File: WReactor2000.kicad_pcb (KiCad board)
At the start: 4 copper layers, 63 x 62.2 mm, 32 parts, among them Q1 BSC026N08NS, U1 LTC4359-MS8, U2 ET60T-02-24-02-X-RTX-GP, U4 TM4C1230H6PM, U6 LTC3604_UD, U7 LTC3604_UD

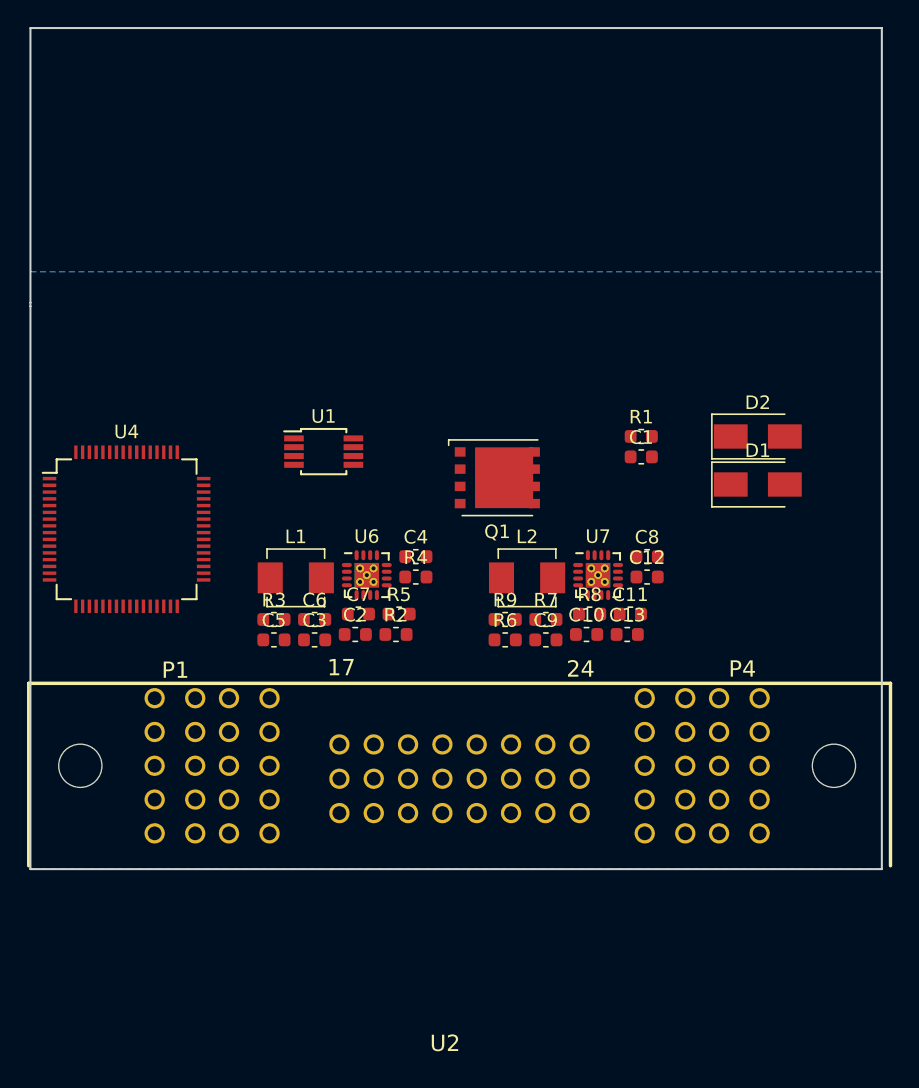
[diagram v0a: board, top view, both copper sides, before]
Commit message: dumb-updates
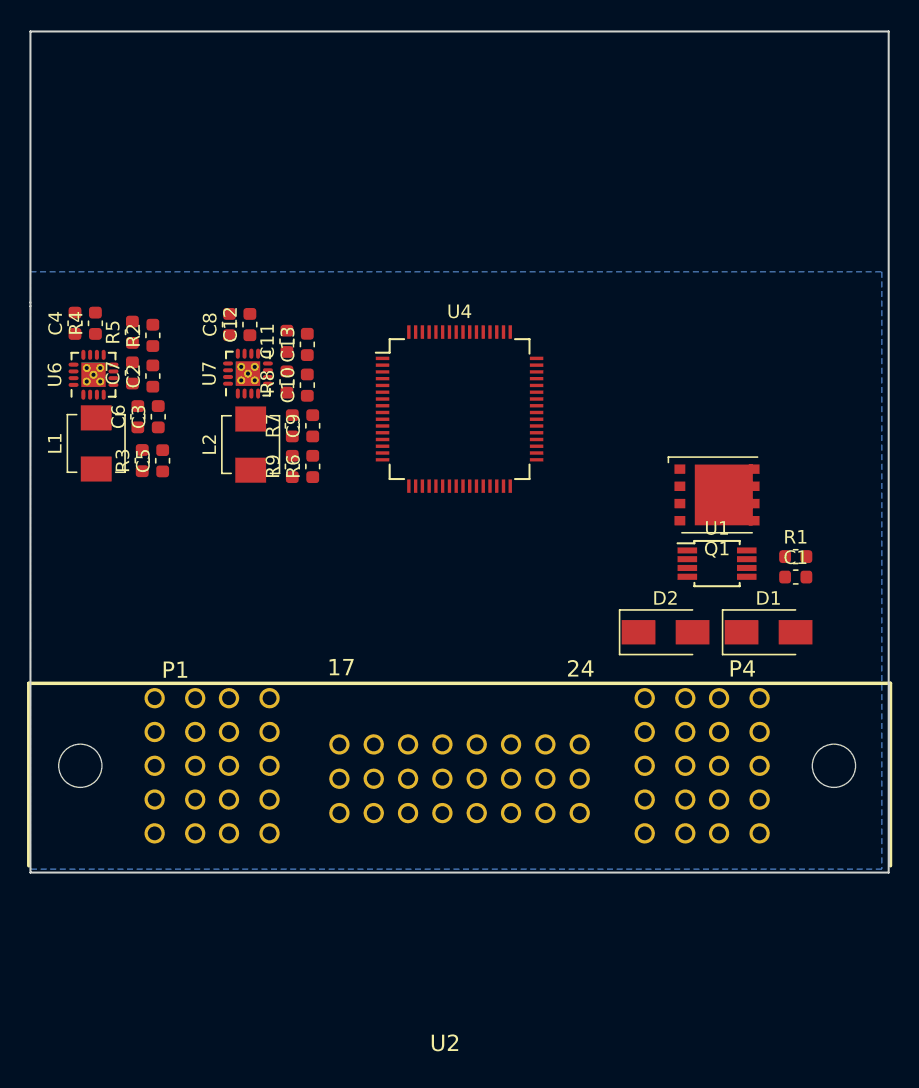
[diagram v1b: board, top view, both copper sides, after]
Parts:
- moved C8 35.3 mm to (65.5, 85.2), turned to 90 degrees
- moved C12 34.8 mm to (67.0, 85.2), turned to 90 degrees
- moved C11 32.4 mm to (69.8, 86.4), turned to 90 degrees
- moved C13 31.9 mm to (71.3, 86.7), turned to 90 degrees
- moved C4 30.6 mm to (54.1, 85.1), turned to 90 degrees
- moved U1 30.3 mm to (101.6, 102.9)
- moved R4 30.2 mm to (55.6, 85.1), turned to 90 degrees
- moved U7 29.9 mm to (66.9, 88.8), turned to 90 degrees
- moved R5 28.7 mm to (58.3, 85.8), turned to 90 degrees
- moved R2 28.5 mm to (59.9, 86.0), turned to 90 degrees
- moved R8 28.2 mm to (69.8, 89.4), turned to 90 degrees
- moved C10 27.7 mm to (71.3, 89.7), turned to 90 degrees
- moved U4 26.2 mm to (82.5, 91.4)
- moved U6 25.1 mm to (55.5, 88.9), turned to 90 degrees
- moved C7 24.5 mm to (58.3, 88.8), turned to 90 degrees
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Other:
- board size 63 x 62.2 mm -> 63.5 x 62.2 mm
